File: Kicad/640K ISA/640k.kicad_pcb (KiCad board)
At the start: 2 copper layers, 104 x 73.9 mm, 17 parts, among them J9 Bus_ISA_8bit, U1 62256, U2 28C256, U3 AS6C4008, U4 74LS139, U5 74LS138, U6 AS6C1008

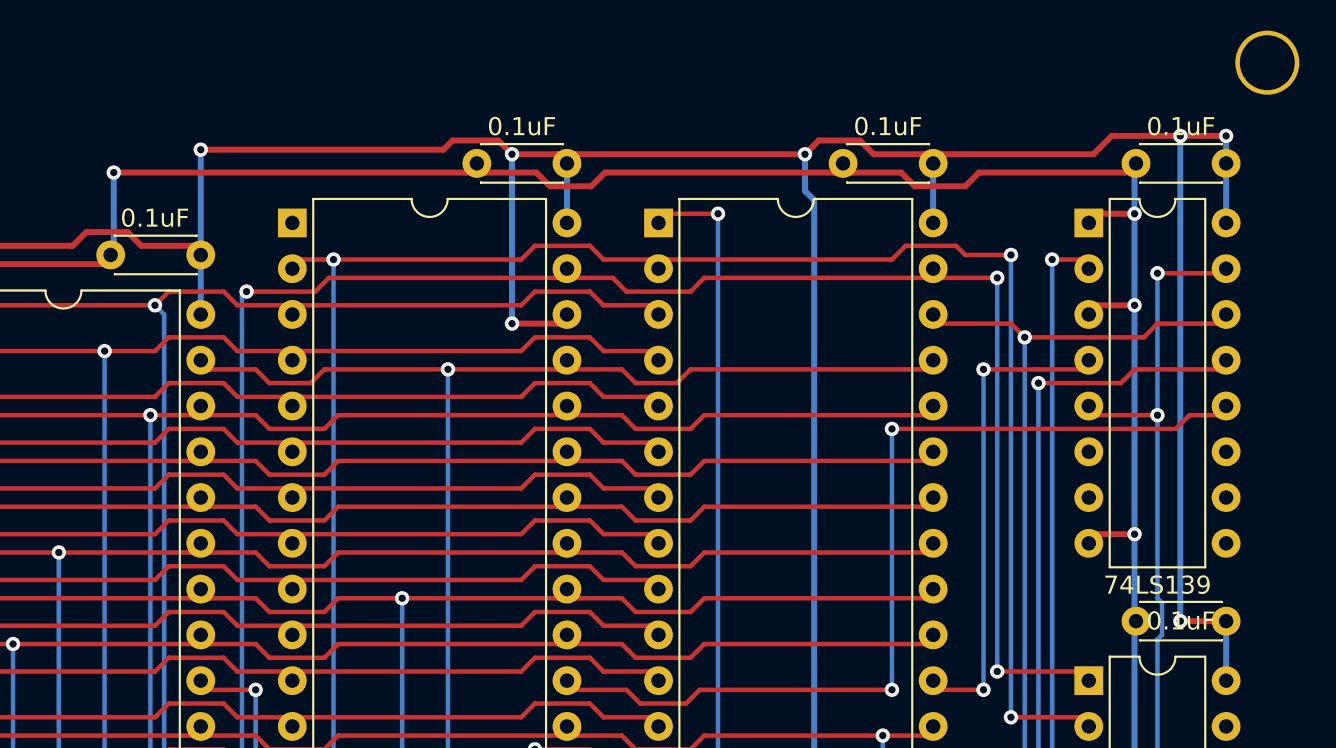
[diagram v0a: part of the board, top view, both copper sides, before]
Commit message: 640k update
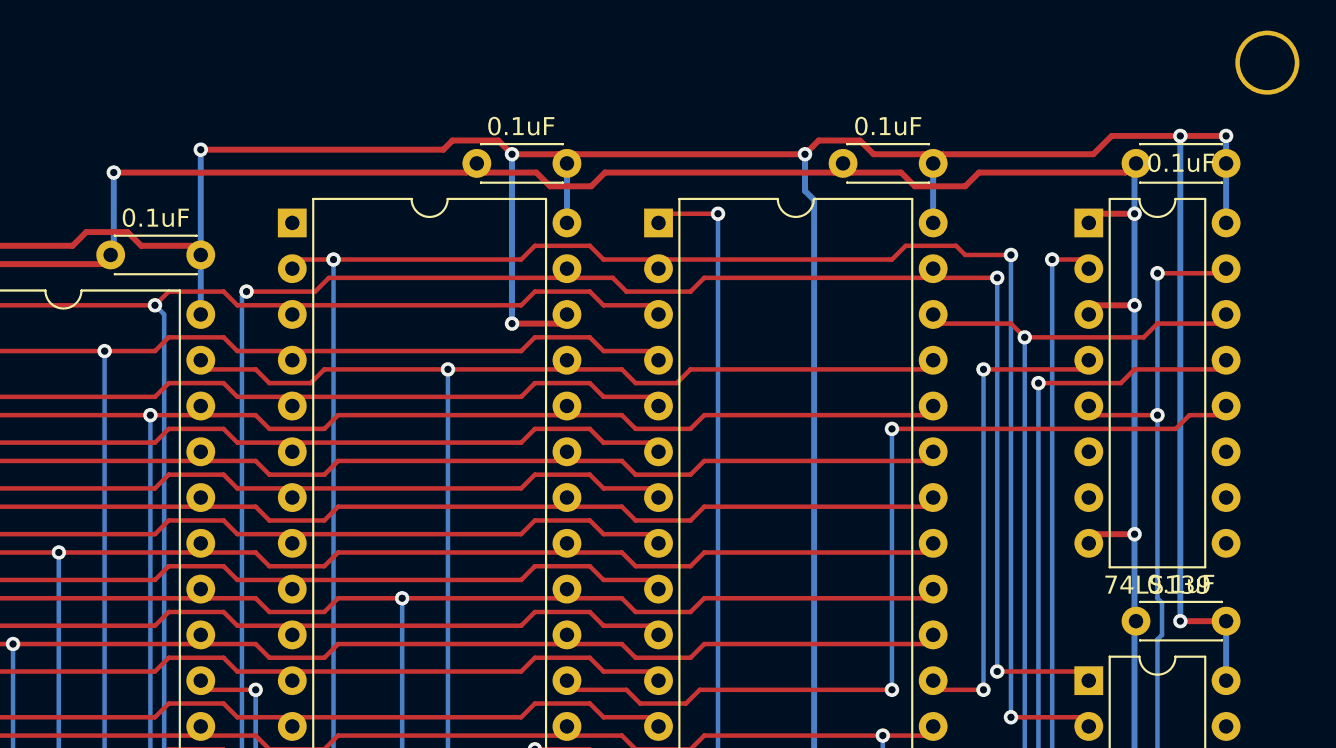
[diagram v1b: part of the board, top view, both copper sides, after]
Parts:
- moved C6 30.2 mm to (174.3, 96.0)
- moved C5 25.4 mm to (174.3, 70.6)
- moved C2 20.9 mm to (117.4, 75.7)
- moved C3 20.9 mm to (137.7, 70.6)
- moved C4 16.3 mm to (158.1, 70.6)
- renumbered U2 to U1, U1 to U2, U6 to U3, U3 to U4, U4 to U5, U5 to U6
